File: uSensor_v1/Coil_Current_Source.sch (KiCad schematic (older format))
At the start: 12 parts, among them Q3 Q_NPN_BCE, Q4 Q_PNP_BCE, U17 LM6132A/NS

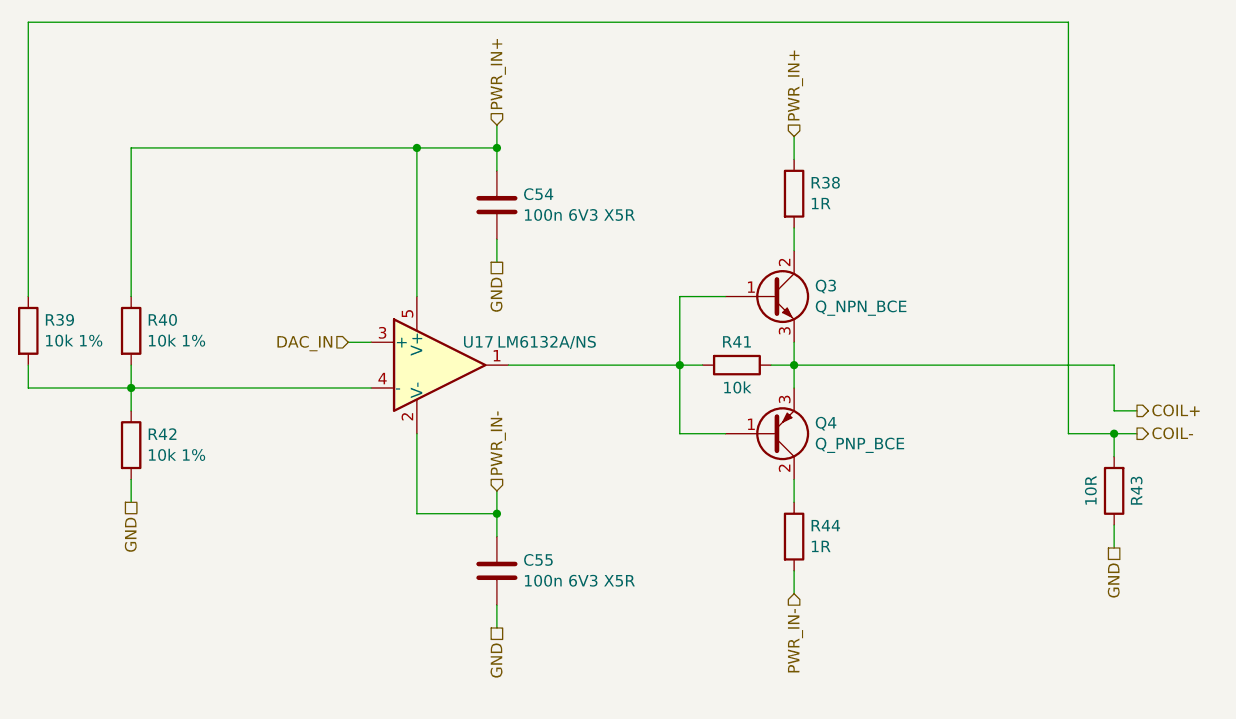
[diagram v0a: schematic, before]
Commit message: Schematic in progress.
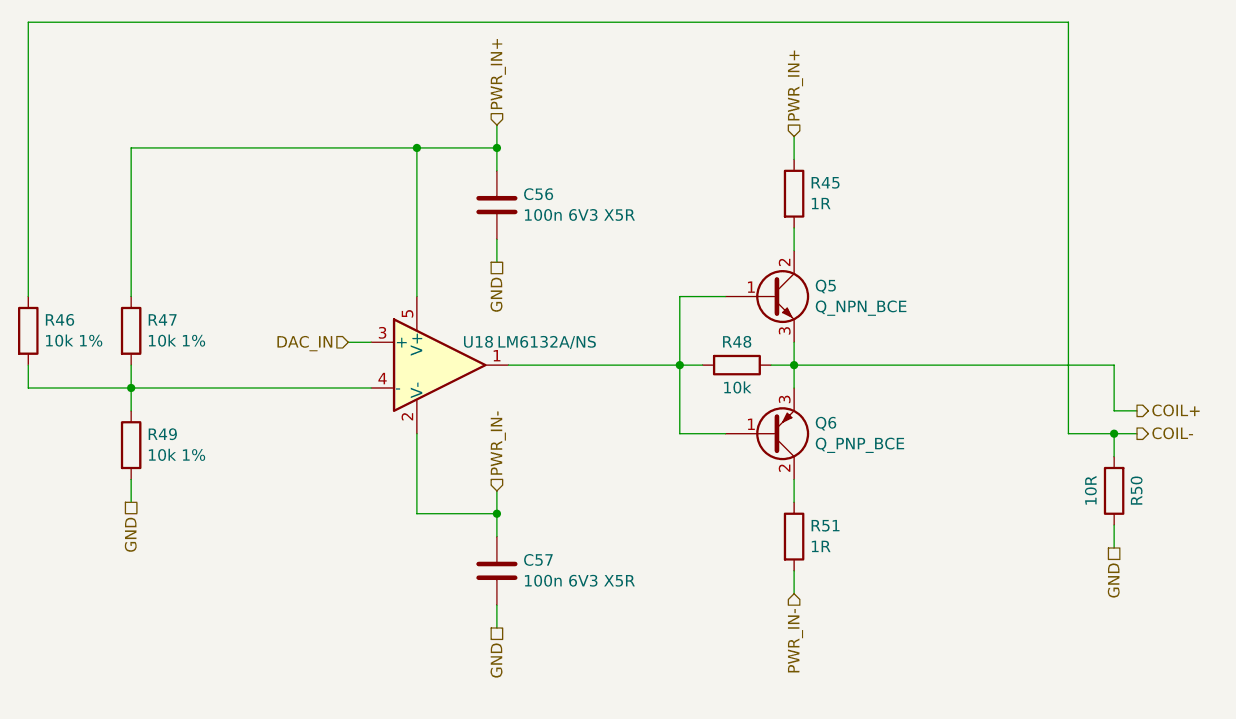
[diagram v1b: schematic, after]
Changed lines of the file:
@@
 $Descr A4 11693 8268
 encoding utf-8
-Sheet 3 7
+Sheet 4 7
 Title ""
 Date ""
@@
 AR Path="/5C398D6C/5C48099D" Ref="U17"  Part="1"
 AR Path="/5C839FF6/5C48099D" Ref="U18"  Part="1"
-F 0 "U17" H 5350 3800 50  0000 L CNN
+F 0 "U18" H 5350 3800 50  0000 L CNN
 F 1 "LM6132A/NS" H 5500 3800 50  0000 L CNN
 F 2 "" H 5250 3700 50  0001 C CNN
@@
 AR Path="/5C398D6C/5C4809A6" Ref="C54"  Part="1"
 AR Path="/5C839FF6/5C4809A6" Ref="C56"  Part="1"
-F 0 "C54" H 5615 3046 50  0000 L CNN
+F 0 "C56" H 5615 3046 50  0000 L CNN
 F 1 "100n 6V3 X5R" H 5615 2955 50  0000 L CNN
 F 2 "Capacitor_SMD:C_0603_1608Metric_Pad1.05x0.95mm_HandSolder" H 5538 2850 50  0001 C CNN
@@
 AR Path="/5C398D6C/5C4809BF" Ref="C55"  Part="1"
 AR Path="/5C839FF6/5C4809BF" Ref="C57"  Part="1"
-F 0 "C55" H 5615 4646 50  0000 L CNN
+F 0 "C57" H 5615 4646 50  0000 L CNN
 F 1 "100n 6V3 X5R" H 5615 4555 50  0000 L CNN
 F 2 "Capacitor_SMD:C_0603_1608Metric_Pad1.05x0.95mm_HandSolder" H 5538 4450 50  0001 C CNN
@@
 AR Path="/5C398D6C/5C4809DE" Ref="R42"  Part="1"
 AR Path="/5C839FF6/5C4809DE" Ref="R49"  Part="1"
-F 0 "R42" H 3970 4096 50  0000 L CNN
+F 0 "R49" H 3970 4096 50  0000 L CNN
 F 1 "10k 1%" H 3970 4005 50  0000 L CNN
 F 2 "Resistor_SMD:R_0603_1608Metric_Pad1.05x0.95mm_HandSolder" V 3830 4050 50  0001 C CNN
@@
 AR Path="/5C398D6C/5C4809E6" Ref="R40"  Part="1"
 AR Path="/5C839FF6/5C4809E6" Ref="R47"  Part="1"
-F 0 "R40" H 3970 3596 50  0000 L CNN
+F 0 "R47" H 3970 3596 50  0000 L CNN
 F 1 "10k 1%" H 3970 3505 50  0000 L CNN
 F 2 "Resistor_SMD:R_0603_1608Metric_Pad1.05x0.95mm_HandSolder" V 3830 3550 50  0001 C CNN
@@
 AR Path="/5C398D6C/5C4809ED" Ref="R39"  Part="1"
 AR Path="/5C839FF6/5C4809ED" Ref="R46"  Part="1"
-F 0 "R39" H 3520 3596 50  0000 L CNN
+F 0 "R46" H 3520 3596 50  0000 L CNN
 F 1 "10k 1%" H 3520 3505 50  0000 L CNN
 F 2 "Resistor_SMD:R_0603_1608Metric_Pad1.05x0.95mm_HandSolder" V 3380 3550 50  0001 C CNN
@@
 AR Path="/5C398D6C/5C4809FD" Ref="Q3"  Part="1"
 AR Path="/5C839FF6/5C4809FD" Ref="Q5"  Part="1"
-F 0 "Q3" H 6891 3446 50  0000 L CNN
+F 0 "Q5" H 6891 3446 50  0000 L CNN
 F 1 "Q_NPN_BCE" H 6891 3355 50  0000 L CNN
 F 2 "" H 6900 3500 50  0001 C CNN
@@
 AR Path="/5C398D6C/5C480A04" Ref="Q4"  Part="1"
 AR Path="/5C839FF6/5C480A04" Ref="Q6"  Part="1"
-F 0 "Q4" H 6891 3954 50  0000 L CNN
+F 0 "Q6" H 6891 3954 50  0000 L CNN
 F 1 "Q_PNP_BCE" H 6891 4045 50  0000 L CNN
 F 2 "" H 6900 4100 50  0001 C CNN
@@
 AR Path="/5C398D6C/5C480A0B" Ref="R41"  Part="1"
 AR Path="/5C839FF6/5C480A0B" Ref="R48"  Part="1"
-F 0 "R41" V 6450 3700 50  0000 C CNN
+F 0 "R48" V 6450 3700 50  0000 C CNN
 F 1 "10k" V 6650 3700 50  0000 C CNN
 F 2 "Resistor_SMD:R_0603_1608Metric_Pad1.05x0.95mm_HandSolder" V 6480 3700 50  0001 C CNN
@@
 AR Path="/5C398D6C/5C480A1D" Ref="R38"  Part="1"
 AR Path="/5C839FF6/5C480A1D" Ref="R45"  Part="1"
-F 0 "R38" H 6870 2996 50  0000 L CNN
+F 0 "R45" H 6870 2996 50  0000 L CNN
 F 1 "1R" H 6870 2905 50  0000 L CNN
 F 2 "Resistor_SMD:R_0603_1608Metric_Pad1.05x0.95mm_HandSolder" V 6730 2950 50  0001 C CNN
@@
 AR Path="/5C398D6C/5C480A25" Ref="R44"  Part="1"
 AR Path="/5C839FF6/5C480A25" Ref="R51"  Part="1"
-F 0 "R44" H 6870 4496 50  0000 L CNN
+F 0 "R51" H 6870 4496 50  0000 L CNN
 F 1 "1R" H 6870 4405 50  0000 L CNN
 F 2 "Resistor_SMD:R_0603_1608Metric_Pad1.05x0.95mm_HandSolder" V 6730 4450 50  0001 C CNN
@@
 AR Path="/5C398D6C/5C480A49" Ref="R43"  Part="1"
 AR Path="/5C839FF6/5C480A49" Ref="R50"  Part="1"
-F 0 "R43" V 8100 4250 50  0000 C CNN
+F 0 "R50" V 8100 4250 50  0000 C CNN
 F 1 "10R" V 8300 4250 50  0000 C CNN
 F 2 "Resistor_SMD:R_0603_1608Metric_Pad1.05x0.95mm_HandSolder" V 8130 4250 50  0001 C CNN

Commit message: Schematic in progress.
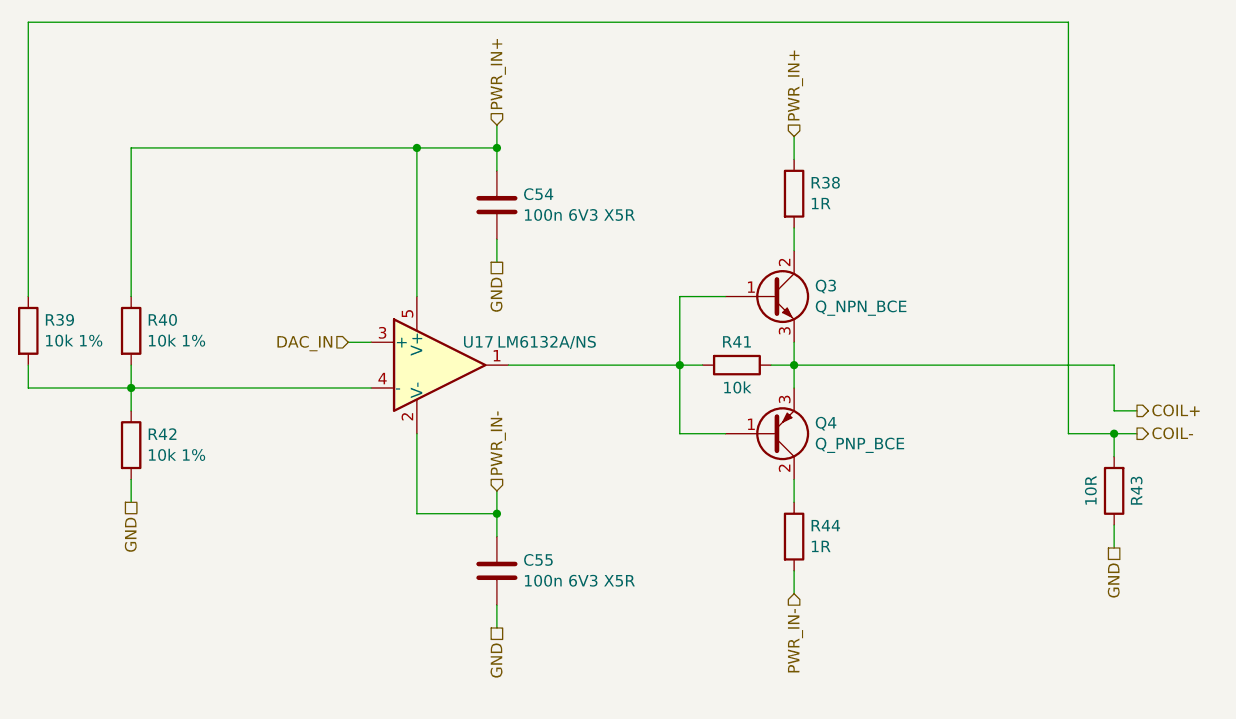
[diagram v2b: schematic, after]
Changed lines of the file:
@@
 $Descr A4 11693 8268
 encoding utf-8
-Sheet 4 7
+Sheet 3 7
 Title ""
 Date ""
@@
 AR Path="/5C398D6C/5C48099D" Ref="U17"  Part="1"
 AR Path="/5C839FF6/5C48099D" Ref="U18"  Part="1"
-F 0 "U18" H 5350 3800 50  0000 L CNN
+F 0 "U17" H 5350 3800 50  0000 L CNN
 F 1 "LM6132A/NS" H 5500 3800 50  0000 L CNN
 F 2 "" H 5250 3700 50  0001 C CNN
@@
 AR Path="/5C398D6C/5C4809A6" Ref="C54"  Part="1"
 AR Path="/5C839FF6/5C4809A6" Ref="C56"  Part="1"
-F 0 "C56" H 5615 3046 50  0000 L CNN
+F 0 "C54" H 5615 3046 50  0000 L CNN
 F 1 "100n 6V3 X5R" H 5615 2955 50  0000 L CNN
 F 2 "Capacitor_SMD:C_0603_1608Metric_Pad1.05x0.95mm_HandSolder" H 5538 2850 50  0001 C CNN
@@
 AR Path="/5C398D6C/5C4809BF" Ref="C55"  Part="1"
 AR Path="/5C839FF6/5C4809BF" Ref="C57"  Part="1"
-F 0 "C57" H 5615 4646 50  0000 L CNN
+F 0 "C55" H 5615 4646 50  0000 L CNN
 F 1 "100n 6V3 X5R" H 5615 4555 50  0000 L CNN
 F 2 "Capacitor_SMD:C_0603_1608Metric_Pad1.05x0.95mm_HandSolder" H 5538 4450 50  0001 C CNN
@@
 AR Path="/5C398D6C/5C4809DE" Ref="R42"  Part="1"
 AR Path="/5C839FF6/5C4809DE" Ref="R49"  Part="1"
-F 0 "R49" H 3970 4096 50  0000 L CNN
+F 0 "R42" H 3970 4096 50  0000 L CNN
 F 1 "10k 1%" H 3970 4005 50  0000 L CNN
 F 2 "Resistor_SMD:R_0603_1608Metric_Pad1.05x0.95mm_HandSolder" V 3830 4050 50  0001 C CNN
@@
 AR Path="/5C398D6C/5C4809E6" Ref="R40"  Part="1"
 AR Path="/5C839FF6/5C4809E6" Ref="R47"  Part="1"
-F 0 "R47" H 3970 3596 50  0000 L CNN
+F 0 "R40" H 3970 3596 50  0000 L CNN
 F 1 "10k 1%" H 3970 3505 50  0000 L CNN
 F 2 "Resistor_SMD:R_0603_1608Metric_Pad1.05x0.95mm_HandSolder" V 3830 3550 50  0001 C CNN
@@
 AR Path="/5C398D6C/5C4809ED" Ref="R39"  Part="1"
 AR Path="/5C839FF6/5C4809ED" Ref="R46"  Part="1"
-F 0 "R46" H 3520 3596 50  0000 L CNN
+F 0 "R39" H 3520 3596 50  0000 L CNN
 F 1 "10k 1%" H 3520 3505 50  0000 L CNN
 F 2 "Resistor_SMD:R_0603_1608Metric_Pad1.05x0.95mm_HandSolder" V 3380 3550 50  0001 C CNN
@@
 AR Path="/5C398D6C/5C4809FD" Ref="Q3"  Part="1"
 AR Path="/5C839FF6/5C4809FD" Ref="Q5"  Part="1"
-F 0 "Q5" H 6891 3446 50  0000 L CNN
+F 0 "Q3" H 6891 3446 50  0000 L CNN
 F 1 "Q_NPN_BCE" H 6891 3355 50  0000 L CNN
 F 2 "" H 6900 3500 50  0001 C CNN
@@
 AR Path="/5C398D6C/5C480A04" Ref="Q4"  Part="1"
 AR Path="/5C839FF6/5C480A04" Ref="Q6"  Part="1"
-F 0 "Q6" H 6891 3954 50  0000 L CNN
+F 0 "Q4" H 6891 3954 50  0000 L CNN
 F 1 "Q_PNP_BCE" H 6891 4045 50  0000 L CNN
 F 2 "" H 6900 4100 50  0001 C CNN
@@
 AR Path="/5C398D6C/5C480A0B" Ref="R41"  Part="1"
 AR Path="/5C839FF6/5C480A0B" Ref="R48"  Part="1"
-F 0 "R48" V 6450 3700 50  0000 C CNN
+F 0 "R41" V 6450 3700 50  0000 C CNN
 F 1 "10k" V 6650 3700 50  0000 C CNN
 F 2 "Resistor_SMD:R_0603_1608Metric_Pad1.05x0.95mm_HandSolder" V 6480 3700 50  0001 C CNN
@@
 AR Path="/5C398D6C/5C480A1D" Ref="R38"  Part="1"
 AR Path="/5C839FF6/5C480A1D" Ref="R45"  Part="1"
-F 0 "R45" H 6870 2996 50  0000 L CNN
+F 0 "R38" H 6870 2996 50  0000 L CNN
 F 1 "1R" H 6870 2905 50  0000 L CNN
 F 2 "Resistor_SMD:R_0603_1608Metric_Pad1.05x0.95mm_HandSolder" V 6730 2950 50  0001 C CNN
@@
 AR Path="/5C398D6C/5C480A25" Ref="R44"  Part="1"
 AR Path="/5C839FF6/5C480A25" Ref="R51"  Part="1"
-F 0 "R51" H 6870 4496 50  0000 L CNN
+F 0 "R44" H 6870 4496 50  0000 L CNN
 F 1 "1R" H 6870 4405 50  0000 L CNN
 F 2 "Resistor_SMD:R_0603_1608Metric_Pad1.05x0.95mm_HandSolder" V 6730 4450 50  0001 C CNN
@@
 AR Path="/5C398D6C/5C480A49" Ref="R43"  Part="1"
 AR Path="/5C839FF6/5C480A49" Ref="R50"  Part="1"
-F 0 "R50" V 8100 4250 50  0000 C CNN
+F 0 "R43" V 8100 4250 50  0000 C CNN
 F 1 "10R" V 8300 4250 50  0000 C CNN
 F 2 "Resistor_SMD:R_0603_1608Metric_Pad1.05x0.95mm_HandSolder" V 8130 4250 50  0001 C CNN
